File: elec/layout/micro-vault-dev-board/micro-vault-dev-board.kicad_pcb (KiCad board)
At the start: 2 copper layers, 32.3 x 64.4 mm, 39 parts

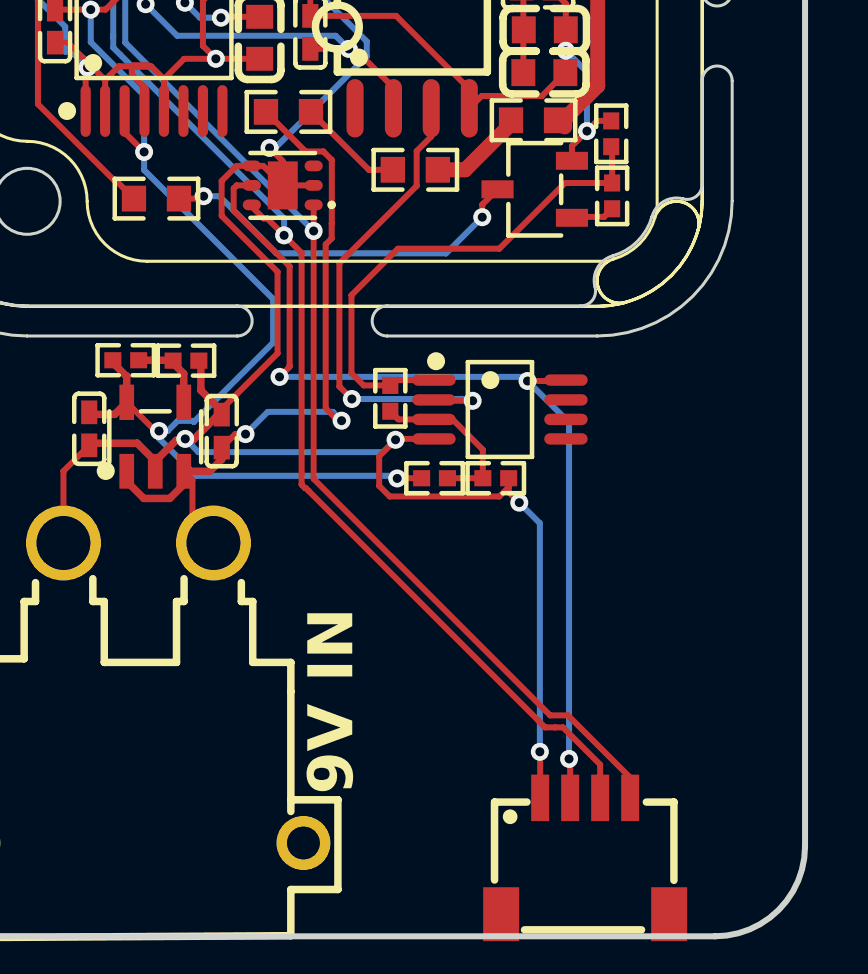
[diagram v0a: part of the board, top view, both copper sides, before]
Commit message: update layout
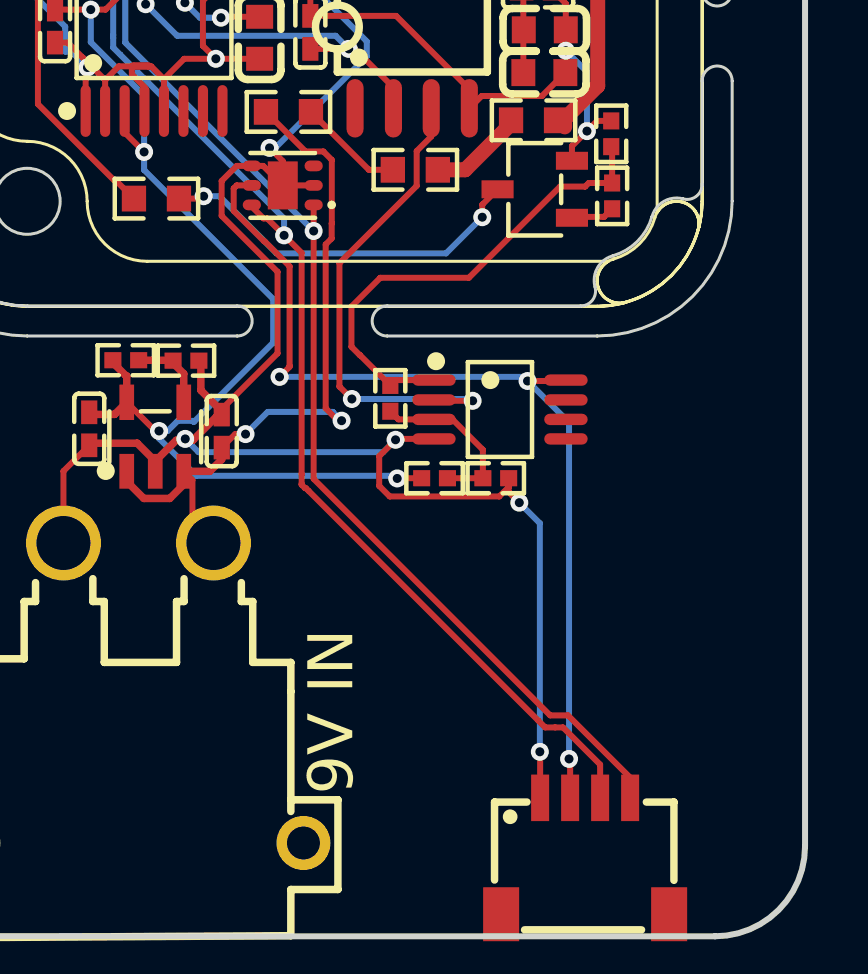
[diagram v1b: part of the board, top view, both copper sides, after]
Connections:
- net TEMP renamed IN1minus
- C1 pad 1: hv -> hv-1
- C1 pad 2: gnd -> gnd-1
- C10 pad 2: gnd -> gnd-1
- C2 pad 1: hv -> hv-1
- C2 pad 2: gnd -> gnd-1
- C3 pad 1: hv-1 -> hv-2
- C4 pad 1: hv-1 -> hv-2
- C5 pad 1: hv-2 -> hv-3
- C6 pad 1: hv-2 -> hv-3
- C7 pad 1: hv-2 -> hv-3
- C8 pad 1: hv-3 -> hv
- C9 pad 1: hv-1 -> hv-2
- J1 pad 2: hv-3 -> hv
- R13 pad 1: hv-1 -> hv-2
- R15 pad 1: hv-1 -> hv-2
- R17 pad 1: gnd -> gnd-1
- R17 pad 2: gnd-1 -> gnd
- R2 pad 1: hv-3 -> hv
- R2 pad 2: micro_vault.heater_controller-net-5 -> micro_vault.heater_controller-net-1
- R3 pad 1: micro_vault.heater_controller-net-5 -> micro_vault.heater_controller-net-1
- R3 pad 2: micro_vault.heater_controller-net-6 -> micro_vault.heater_controller-net-3
- R4 pad 1: micro_vault.heater_controller-net-6 -> micro_vault.heater_controller-net-3
- R4 pad 2: micro_vault.heater_controller-net-2 -> micro_vault.heater_controller-net-4
- R5 pad 1: micro_vault.heater_controller-net-2 -> micro_vault.heater_controller-net-4
- R5 pad 2: micro_vault.heater_controller-net-4 -> micro_vault.heater_controller-net-6
- R6 pad 1: micro_vault.heater_controller-net-4 -> micro_vault.heater_controller-net-6
- R6 pad 2: micro_vault.heater_controller-net-1 -> micro_vault.heater_controller-net
- R7 pad 1: micro_vault.heater_controller-net-1 -> micro_vault.heater_controller-net
- R7 pad 2: micro_vault.heater_controller-net-3 -> micro_vault.heater_controller-net-2
- R8 pad 1: micro_vault.heater_controller-net-3 -> micro_vault.heater_controller-net-2
- R8 pad 2: micro_vault.heater_controller-net -> micro_vault.heater_controller-net-5
- R9 pad 1: micro_vault.heater_controller-net -> micro_vault.heater_controller-net-5
- U1 pad 1: gnd-1 -> gnd
- U1 pad 2: gnd-1 -> gnd
- U3 pad 2: gnd -> gnd-1
- U4 pad 1: hv -> hv-1
- U4 pad 2: hv-1 -> hv-2
- U5 pad 12: hv -> hv-1
- U5 pad 13: hv-1 -> hv-2
- U5 pad 3: hv-1 -> hv-2
- U5 pad 5: gnd -> gnd-1
- U5 pad 9: gnd -> gnd-1
- U7 pad 2: hv-1 -> hv-2
- U7 pad 6: hv-2 -> hv-3
- U8 pad 1: hv-3 -> hv
- U8 pad 3: hv-3 -> hv
- U8 pad 5: hv-1 -> hv-2
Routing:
- net hv-2: track 7.05 -> 51.8 mm, vias 0 -> 6
- net hv-1: track 51.8 -> 7.33 mm, vias 6 -> 2
- net hv-3: track 24.3 -> 7.05 mm, vias 2 -> 0
- net hv: track 7.33 -> 24.3 mm
- net gnd-1: track 28.4 -> 19.6 mm, vias 0 -> 3
- net gnd: track 19.6 -> 28.4 mm, vias 3 -> 0
- net micro_vault.heater_controller-net-3: track 10.5 -> 2.93 mm, vias 2 -> 0
- net micro_vault.heater_controller-net-5: track 3.53 -> 9.44 mm
- net micro_vault.heater_controller-net: track 9.44 -> 3.70 mm
- net micro_vault.heater_controller-net-4: track 3.89 -> 7.27 mm
- net micro_vault.heater_controller-net-2: track 7.27 -> 10.5 mm, vias 0 -> 2
- net micro_vault.heater_controller-net-6: track 2.93 -> 3.89 mm

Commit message: building frozen
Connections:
- net hv-4 renamed line-1
- C1 pad 1: hv-1 -> hv
- C2 pad 1: hv-1 -> hv
- C3 pad 1: hv-2 -> hv-3
- C3 pad 2: gnd-2 -> gnd-1
- C4 pad 1: hv-2 -> hv-3
- C4 pad 2: gnd-2 -> gnd-1
- C5 pad 1: hv-3 -> hv-2
- C5 pad 2: gnd-2 -> gnd-1
- C6 pad 1: hv-3 -> hv-2
- C6 pad 2: gnd-2 -> gnd-1
- C7 pad 1: hv-3 -> hv-2
- C7 pad 2: gnd-2 -> gnd-1
- C8 pad 1: hv -> hv-1
- C8 pad 2: gnd-2 -> gnd-1
- C9 pad 1: hv-2 -> hv-3
- C9 pad 2: gnd-2 -> gnd-1
- J1 pad 1: gnd-2 -> gnd-1
- J1 pad 2: hv -> hv-1
- Q1 pad 2: gnd-2 -> gnd-1
- R11 pad 2: gnd-2 -> gnd-1
- R12 pad 2: gnd-2 -> gnd-1
- R13 pad 1: hv-2 -> hv-3
- R14 pad 2: gnd-2 -> gnd-1
- R15 pad 1: hv-2 -> hv-3
- R2 pad 1: hv -> hv-1
- R2 pad 2: micro_vault.heater_controller-net-1 -> micro_vault.heater_controller-net-3
- R3 pad 1: micro_vault.heater_controller-net-1 -> micro_vault.heater_controller-net-3
- R3 pad 2: micro_vault.heater_controller-net-3 -> micro_vault.heater_controller-net-5
- R4 pad 1: micro_vault.heater_controller-net-3 -> micro_vault.heater_controller-net-5
- R5 pad 2: micro_vault.heater_controller-net-6 -> micro_vault.heater_controller-net-1
- R6 pad 1: micro_vault.heater_controller-net-6 -> micro_vault.heater_controller-net-1
- R8 pad 2: micro_vault.heater_controller-net-5 -> micro_vault.heater_controller-net-6
- R9 pad 1: micro_vault.heater_controller-net-5 -> micro_vault.heater_controller-net-6
- U3 pad 1: gnd-2 -> gnd-1
- U4 pad 1: hv-1 -> hv
- U4 pad 2: hv-2 -> hv-3
- U5 pad 1: gnd-2 -> gnd-1
- U5 pad 12: hv-1 -> hv
- U5 pad 13: hv-2 -> hv-3
- U5 pad 2: gnd-2 -> gnd-1
- U5 pad 3: hv-2 -> hv-3
- U5 pad 4: gnd-2 -> gnd-1
- U5 pad 8: REFN -> hv-2
- U6 pad 4: gnd-2 -> gnd-1
- U7 pad 2: hv-2 -> hv-3
- U7 pad 4: gnd-2 -> gnd-1
- U7 pad 6: hv-3 -> hv-2
- U8 pad 1: hv -> hv-1
- U8 pad 2: gnd-2 -> gnd-1
- U8 pad 3: hv -> hv-1
- U8 pad 5: hv-2 -> hv-3
- U9 pad 2: gnd-2 -> gnd-1
- U9 pad 4: gnd-2 -> gnd-1
- U9 pad 7: gnd-2 -> gnd-1
- X1 pad 1: gnd-2 -> gnd-1
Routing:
- net (no net): track 0.00 -> 133.0 mm, vias 0 -> 12
- net gnd-2: track 106.3 -> 0.00 mm, vias 9 -> 0
- net hv-2: track 51.8 -> 0.00 mm, vias 6 -> 0
- net hv-3: track 7.05 -> 51.8 mm, vias 0 -> 6
- net gnd-1: track 19.6 -> 0.00 mm, vias 3 -> 0
- net hv-1: track 7.33 -> 24.3 mm
- net hv: track 24.3 -> 7.33 mm
- net micro_vault.heater_controller-net-5: track 9.44 -> 2.93 mm
- net micro_vault.heater_controller-net-6: track 3.89 -> 9.44 mm
- net micro_vault.heater_controller-net-3: track 2.93 -> 3.53 mm

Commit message: building locally to fix frozen builds
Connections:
- net IN1minus renamed TEMP
- C1 pad 1: hv -> hv-1
- C2 pad 1: hv -> hv-1
- C3 pad 1: hv-3 -> hv-2
- C4 pad 1: hv-3 -> hv-2
- C5 pad 1: hv-2 -> hv-3
- C6 pad 1: hv-2 -> hv-3
- C7 pad 1: hv-2 -> hv-3
- C8 pad 1: hv-1 -> hv-4
- C9 pad 1: hv-3 -> hv-2
- J1 pad 2: hv-1 -> hv-4
- R13 pad 1: hv-3 -> hv-2
- R15 pad 1: hv-3 -> hv-2
- R16 pad 1: line-1 -> hv
- R2 pad 1: hv-1 -> hv-4
- R2 pad 2: micro_vault.heater_controller-net-3 -> micro_vault.heater_controller-net
- R3 pad 1: micro_vault.heater_controller-net-3 -> micro_vault.heater_controller-net
- R3 pad 2: micro_vault.heater_controller-net-5 -> micro_vault.heater_controller-net-4
- R4 pad 1: micro_vault.heater_controller-net-5 -> micro_vault.heater_controller-net-4
- R4 pad 2: micro_vault.heater_controller-net-4 -> micro_vault.heater_controller-net-6
- R5 pad 1: micro_vault.heater_controller-net-4 -> micro_vault.heater_controller-net-6
- R5 pad 2: micro_vault.heater_controller-net-1 -> micro_vault.heater_controller-net-2
- R6 pad 1: micro_vault.heater_controller-net-1 -> micro_vault.heater_controller-net-2
- R6 pad 2: micro_vault.heater_controller-net -> micro_vault.heater_controller-net-3
- R7 pad 1: micro_vault.heater_controller-net -> micro_vault.heater_controller-net-3
- R7 pad 2: micro_vault.heater_controller-net-2 -> micro_vault.heater_controller-net-5
- R8 pad 1: micro_vault.heater_controller-net-2 -> micro_vault.heater_controller-net-5
- R8 pad 2: micro_vault.heater_controller-net-6 -> micro_vault.heater_controller-net-1
- R9 pad 1: micro_vault.heater_controller-net-6 -> micro_vault.heater_controller-net-1
- U2 pad 1: line-1 -> hv
- U2 pad 2: line-1 -> hv
- U4 pad 1: hv -> hv-1
- U4 pad 2: hv-3 -> hv-2
- U5 pad 12: hv -> hv-1
- U5 pad 13: hv-3 -> hv-2
- U5 pad 3: hv-3 -> hv-2
- U5 pad 8: hv-2 -> hv-3
- U7 pad 2: hv-3 -> hv-2
- U7 pad 6: hv-2 -> hv-3
- U8 pad 1: hv-1 -> hv-4
- U8 pad 3: hv-1 -> hv-4
- U8 pad 5: hv-3 -> hv-2
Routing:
- net hv-3: track 51.8 -> 0.00 mm, vias 6 -> 0
- net hv-2: track 0.00 -> 51.8 mm, vias 0 -> 6
- net line-1: track 30.7 -> 0.00 mm
- net hv-4: track 0.00 -> 24.3 mm, vias 0 -> 2
- net hv: track 7.33 -> 30.7 mm, vias 2 -> 0
- net hv-1: track 24.3 -> 7.33 mm
- net micro_vault.heater_controller-net-5: track 2.93 -> 10.5 mm, vias 0 -> 2
- net micro_vault.heater_controller-net-2: track 10.5 -> 3.89 mm, vias 2 -> 0
- net micro_vault.heater_controller-net-1: track 3.89 -> 9.44 mm
- net micro_vault.heater_controller-net-4: track 7.27 -> 2.93 mm
- net micro_vault.heater_controller-net-6: track 9.44 -> 7.27 mm
